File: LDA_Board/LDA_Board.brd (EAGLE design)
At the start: 47.5 x 68.4 mm, 65 parts, among them IC1 STM32F407ZET, IC3 IS62WV5121655T, K1 B3U-1000P, K2 B3U-1000P, U1 CJT1117-3.3-SOT223, Y1 27.12MHZ

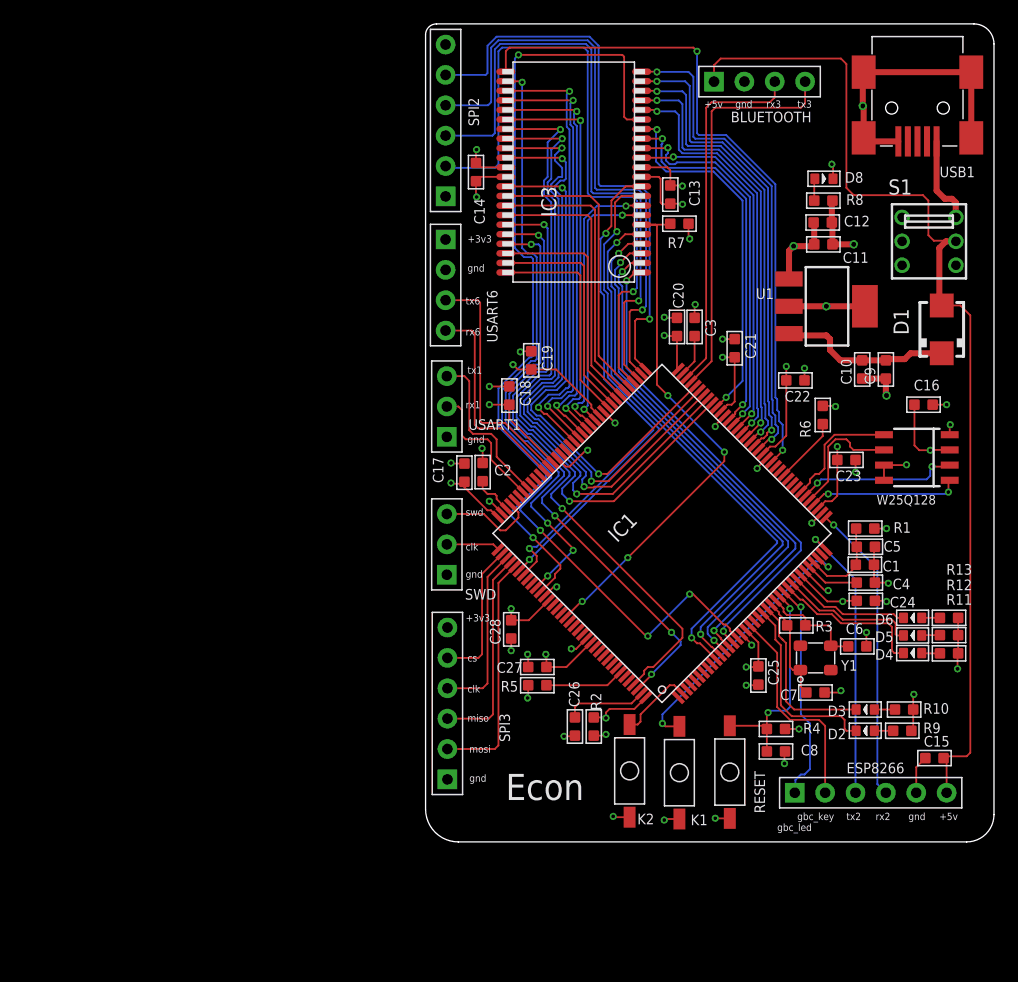
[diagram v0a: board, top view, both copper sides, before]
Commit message: 3D打印了盒子
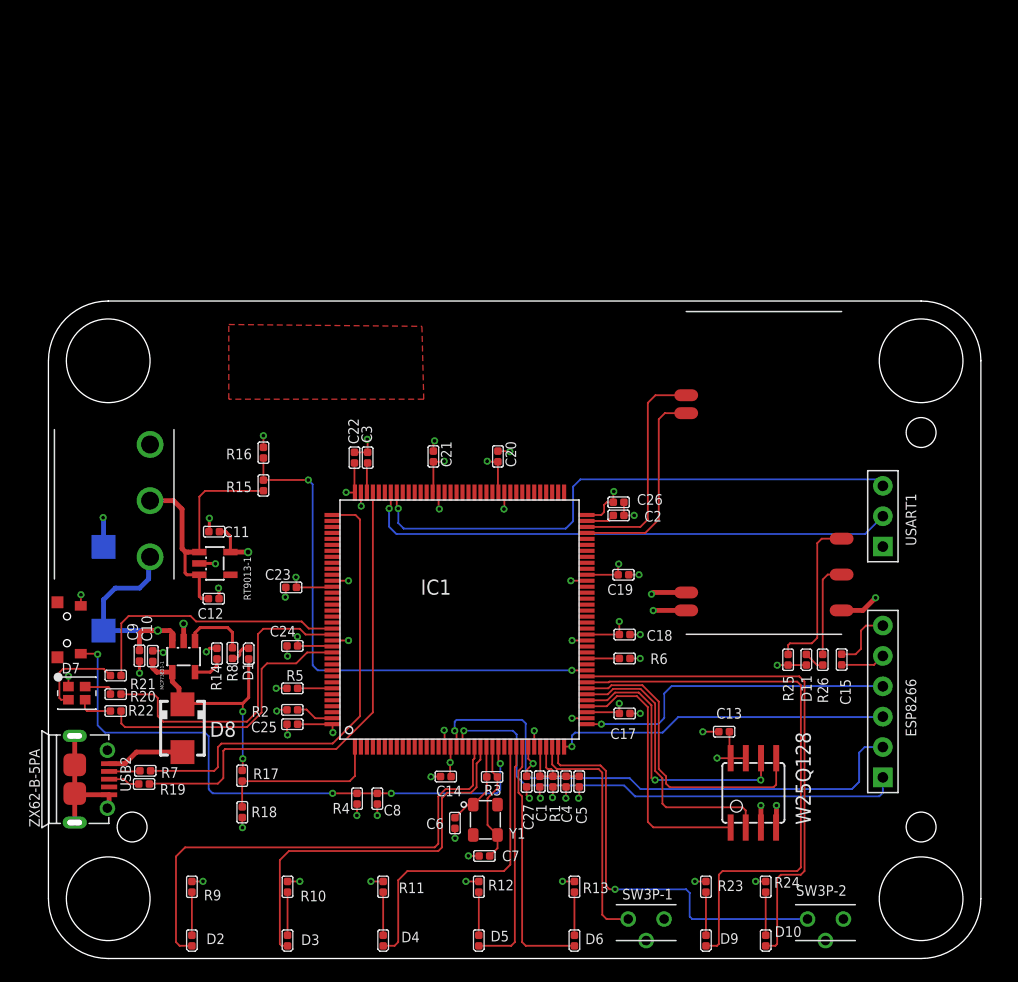
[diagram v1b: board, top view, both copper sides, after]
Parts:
- removed BLUETOOTH, USART6: 4p-2.54, Seeed-OPL-Connector:H4-2.54
- removed C16, C28: 0.5PF 50V, 1-LDA_Board:C0603
- removed IC3: IS62WV5121655T, 1-LDA_Board:TSOP-II-44
- removed K1, K2, RESET: B3U-1000P, 1-LDA_Board:SW2-SMD-3.0X6.0*2.5
- removed S1: 5.8X5.8SWITCH, 1-LDA_Board:2P2T
- removed SPI2, SPI3: 6p-2.54, Seeed-OPL-Connector:H6-2.54
- removed SWD: 3p-2.54, 1-LDA_Board:H3-2.54
- removed U1: CJT1117-3.3-SOT223, 1-LDA_Board:SOT-223
- removed USB1: ST-USB-002A, 1-LDA_Board:MINIUSB5+4P-SMD-0.8-90D
- added B-1: SIDE-BUTTON, 1-LDA_Board:SIDE-BUTTON
- added BATTERY-1: BATTERY, 1-LDA_Board:BATTERY
- added D10, D11, D9: BLUE-0402, 1-LDA_Board:LED-0402
- added D7: HSMF-C118, 1-LDA_Board:LED4-SMD-1210
- added HC05-1: BLUETOOTH, 1-LDA_Board:BLUETOOTH
- added MCP73831-1: MCP73831, 1-LDA_Board:SOT23-5
- added R14: 2k, 1-LDA_Board:R0402
- added R15, R16, R17, R25: 10k, 1-LDA_Board:R0402
- added R18: 20k, 1-LDA_Board:R0402
- added R19: 0R, 1-LDA_Board:R0402
- added R20, R21, R22, R23, R24: 510R, 1-LDA_Board:R0402
- added R26: 1.5k, 1-LDA_Board:R0402
- added RT9013-1: RT9013, 1-LDA_Board:SOT23-5
- added SW-1: SWITCH-3P, 1-LDA_Board:SWITCH-3P
- added SW3P-1, SW3P-2: LD-CCB-001, 1-LDA_Board:SW3-2.54-9.0X3.5X3.5+2.0MM
- added USB2: ZX62-B-5PA, 1-LDA_Board:MICRO-USB5+6P-SMD-0.65-AB
- C1, C13, C14, C2, C3: device 1-LDA_Board:C0603 -> 1-LDA_Board:C0402
- C10, C9: value 0.5PF 50V -> 4.7uf; device 1-LDA_Board:C0603 -> 1-LDA_Board:C0402
- C11: value 0.5PF 50V -> 1uf; device 1-LDA_Board:C0603 -> 1-LDA_Board:C0402
- C12: value 0.5PF 50V -> 10uf; device 1-LDA_Board:C0603 -> 1-LDA_Board:C0402
- C15, C17, C18, C19, C20, C21, C22, C23, C24, C25, C26, C27, C8: value 0.5PF 50V -> 104; device 1-LDA_Board:C0603 -> 1-LDA_Board:C0402
- C4: value 104 -> 10uf; device 1-LDA_Board:C0603 -> 1-LDA_Board:C0402
- C5: value 10uf -> 104; device 1-LDA_Board:C0603 -> 1-LDA_Board:C0402
- C6, C7: value 0.5PF 50V -> 22pf; device 1-LDA_Board:C0603 -> 1-LDA_Board:C0402
- D1: value SS14 -> BLUE-0402; device 1-LDA_Board:SMA -> 1-LDA_Board:LED-0402
- D2, D3, D4, D5, D6: value BLUE-0603 -> BLUE-0402; device Seeed-OPL-Diode:LED-0603 -> 1-LDA_Board:LED-0402
- D8: value BLUE-0603 -> SS14; device Seeed-OPL-Diode:LED-0603 -> 1-LDA_Board:SMA
- R1, R2: device 1-LDA_Board:R0603 -> 1-LDA_Board:R0402
- R10, R11, R12, R13, R9: value 1.1M 1/10W -> 510R; device 1-LDA_Board:R0603 -> 1-LDA_Board:R0402
- R3: value 1.1M 1/10W -> 1M; device 1-LDA_Board:R0603 -> 1-LDA_Board:R0402
- R4: value 1.1M 1/10W -> 10k; device 1-LDA_Board:R0603 -> 1-LDA_Board:R0402
- R5, R6, R7: value 10k -> 0R; device 1-LDA_Board:R0603 -> 1-LDA_Board:R0402
- R8: value 1.1M 1/10W -> 470R; device 1-LDA_Board:R0603 -> 1-LDA_Board:R0402
- W25Q128: device 1-LDA_Board:SOIC8 -> 1-LDA_Board:SOP08
- Y1: value 27.12MHZ -> 8MHZ
- moved D8 70.7 mm to (11.2, 19.3), turned to 270 degrees
- moved C9 66.9 mm to (7.61, 25.3)
- moved D1 64.0 mm to (16.8, 25.5)
- moved C10 64.0 mm to (8.73, 25.3), turned to 0 degrees
- moved R7 64.0 mm to (8.10, 15.7), turned to 90 degrees
- moved R8 62.3 mm to (15.4, 25.5), turned to 180 degrees
- moved R9 60.8 mm to (12.0, 6.00), turned to 0 degrees
- moved C12 59.9 mm to (13.8, 30.1), turned to 270 degrees
- moved D2 59.0 mm to (12.0, 1.50), turned to 270 degrees
- moved C11 56.3 mm to (13.9, 35.7), turned to 270 degrees
- moved R10 53.7 mm to (20.0, 6.00), turned to 0 degrees
- moved D3 52.0 mm to (20.0, 1.50), turned to 270 degrees
- moved R11 51.2 mm to (28.0, 6.00), turned to 0 degrees
- moved C14 50.6 mm to (33.2, 15.2), turned to 90 degrees
- moved D4 50.4 mm to (28.0, 1.50), turned to 270 degrees
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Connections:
- removed net FSMC_A0: IC1.10, IC3.5
- removed net FSMC_A1: IC1.11, IC3.4
- removed net FSMC_A10: IC1.56, IC3.19
- removed net FSMC_A11: IC1.57, IC3.18
- removed net FSMC_A12: IC1.87, IC3.28
- removed net FSMC_A13: IC1.88, IC3.27
- removed net FSMC_A14: IC1.89, IC3.26
- removed net FSMC_A15: IC1.90, IC3.25
- removed net FSMC_A16: IC1.80, IC3.42
- removed net FSMC_A17: IC1.81, IC3.43
- removed net FSMC_A18: IC1.82, IC3.44
- removed net FSMC_A2: IC1.12, IC3.3
- removed net FSMC_A3: IC1.13, IC3.2
- removed net FSMC_A4: IC1.14, IC3.1
- removed net FSMC_A5: IC1.15, IC3.24
- removed net FSMC_A6: IC1.50, IC3.23
- removed net FSMC_A7: IC1.53, IC3.22
- removed net FSMC_A8: IC1.54, IC3.21
- removed net FSMC_A9: IC1.55, IC3.20
- removed net FSMC_D0: IC1.85, IC3.7
- removed net FSMC_D1: IC1.86, IC3.8
- removed net FSMC_D10: IC1.66, IC3.31
- removed net FSMC_D11: IC1.67, IC3.32
- removed net FSMC_D12: IC1.68, IC3.35
- removed net FSMC_D13: IC1.77, IC3.36
- removed net FSMC_D14: IC1.78, IC3.37
- removed net FSMC_D15: IC1.79, IC3.38
- removed net FSMC_D2: IC1.114, IC3.9
- removed net FSMC_D3: IC1.115, IC3.10
- removed net FSMC_D4: IC1.58, IC3.13
- removed net FSMC_D5: IC1.59, IC3.14
- removed net FSMC_D6: IC1.60, IC3.15
- removed net FSMC_D7: IC1.63, IC3.16
- removed net FSMC_D8: IC1.64, IC3.29
- removed net FSMC_D9: IC1.65, IC3.30
- removed net FSMC_NBL0: IC1.141, IC3.39
- removed net FSMC_NBL1: IC1.142, IC3.40
- removed net FSMC_NE3: IC1.125, IC3.6, R7.2
- removed net FSMC_NOE: IC1.118, IC3.41
- removed net FSMC_NWE: IC1.119, IC3.17
- removed net RX6: IC1.97, USART6.4
- removed net SPI2_CLK: IC1.74, SPI2.4
- removed net SPI2_CS: IC1.73, SPI2.5
- removed net SPI2_MISO: IC1.75, SPI2.3
- removed net SPI2_MOSI: IC1.76, SPI2.2
- removed net SPI3_CLK: IC1.111, SPI3.4
- removed net SPI3_CS: IC1.110, SPI3.5
- removed net SPI3_MISO: IC1.112, SPI3.3
- removed net SPI3_MOSI: IC1.113, SPI3.2
- removed net TX6: IC1.96, USART6.3
- new net +3.7V: C12.2, R15.1, RT9013-1.1, RT9013-1.3, SW-1.P$2
- new net BATTERY: BATTERY-1.P$1, C9.2, MCP73831-1.3, SW-1.P$3
- new net LED6: D9.-, IC1.44
- new net LED7: D10.-, IC1.45
- new net LED_B: IC1.129, R20.1
- new net LED_G: IC1.132, R22.1
- new net LED_R: IC1.128, R21.1
- new net LI_CHARGE: IC1.1, R17.2, R18.1
- new net LI_QUANTITY: IC1.46, R15.2, R16.1
- new net N$12: D7.2, R21.2
- new net N$16: D1.-, R8.1
- new net N$17: HC05-1.P$26, R25.1
- new net N$18: D7.3, R22.2
- new net N$19: HC05-1.P$24, R26.1
- new net N$20: D11.+, R26.2
- new net N$24: D9.+, R23.2
- new net N$25: D10.+, R24.2
- new net USB_D+: R19.1, USB2.3
- new net USB_D-: R7.1, USB2.2
- new net VBUS: D8.A, USB2.1
- net +3V3: now also C11.1, C13.2, C14.2, C15.1, ESP8266.6, HC05-1.P$12, R23.1, R24.1, RT9013-1.5, SW3P-1.1; no longer C11.2, C12.2, C13.1, C14.1, C16.1, C28.2, IC3.11, IC3.33, K1.1, R7.1, R8.1, SPI2.6, SPI3.6, U1.2, U1.TER, USART6.1
- net +5V: now also C10.2, D1.+, D8.C, MCP73831-1.4, R17.1; no longer BLUETOOTH.1, C15.1, D1.A, ESP8266.6, S1.2.1
- net CLK: now also R7.2; no longer SWD.2
- net GBC_LED: now also IC1.19; no longer IC1.26
- net GND: now also B-1.P$1, BATTERY-1.P$2, C1.2, C11.2, C13.1, C14.1, C2.2, C3.2, C6.1, C7.1, C8.1, D11.-, D7.1, HC05-1.P$13, HC05-1.P$22, MCP73831-1.2, R14.2, R16.2, R18.2, R25.2, RT9013-1.2, SW3P-2.1, USB2.5, USB2.P1, USB2.P2, USB2.P3, USB2.P4, USB2.P5, USB2.P6; no longer BLUETOOTH.2, C1.1, C11.1, C13.2, C14.2, C16.2, C2.1, C28.1, C3.1, C6.2, C7.2, C8.2, D8.-, IC3.12, IC3.34, K2.1, RESET.2, SPI2.1, SPI3.1, SWD.1, U1.1, USART6.2, USB1.5, USB1.P$1, USB1.P$2, USB1.P$3, USB1.P$4
- net KEY1: now also IC1.35, SW3P-2.2; no longer IC1.2, K2.2
- net N$10: now also D7.4, R20.2; no longer S1.1.1, USB1.1
- net N$11: now also MCP73831-1.5, R14.1; no longer D8.+, R8.2
- net N$2: now also C2.1; no longer C3.2
- net N$3: now also C3.1; no longer C2.2
- net N$4: now also IC1.48; no longer IC1.47
- net N$5: now also C1.1; no longer C1.2
- net N$6: now also MCP73831-1.1, R8.2; no longer C10.2, C9.2, D1.C, U1.3
- net OSC_IN: now also C6.2; no longer C7.1
- net OSC_OUT: now also C7.2; no longer C6.1
- net RESET: now also B-1.P$2, C8.2; no longer C8.1, RESET.1
- net RX3: now also HC05-1.P$1; no longer BLUETOOTH.3
- net SWD: now also R19.2; no longer SWD.3
- net TX3: now also HC05-1.P$2; no longer BLUETOOTH.4
- net WK_UP: now also SW3P-1.2; no longer K1.2
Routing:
- net FSMC_NWE: track 68.0 -> 0.00 mm, vias 2 -> 0
- net FSMC_A5: track 67.7 -> 0.00 mm, vias 4 -> 0
- net +5V: track 87.2 -> 20.0 mm, vias 0 -> 2
- net FSMC_A6: track 57.1 -> 0.00 mm, vias 2 -> 0
- net FSMC_D8: track 56.4 -> 0.00 mm, vias 2 -> 0
- net SPI2_MOSI: track 54.9 -> 0.00 mm, vias 1 -> 0
- net FSMC_D9: track 53.8 -> 0.00 mm, vias 2 -> 0
- net FSMC_NBL0: track 52.7 -> 0.00 mm, vias 2 -> 0
- net SPI2_MISO: track 52.6 -> 0.00 mm, vias 1 -> 0
- net FSMC_D10: track 51.8 -> 0.00 mm, vias 2 -> 0
- net FSMC_NBL1: track 51.6 -> 0.00 mm, vias 4 -> 0
- net SPI2_CLK: track 50.3 -> 0.00 mm, vias 1 -> 0
- net FSMC_D11: track 48.9 -> 0.00 mm, vias 2 -> 0
- net SPI2_CS: track 48.1 -> 0.00 mm, vias 1 -> 0
- net LED6: track 0.00 -> 47.4 mm
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- added copper zone on layer 1, net N$21
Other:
- board size 47.5 x 68.4 mm -> 78 x 55 mm
- board text added: "5个手势显示灯"
- board text added: "ECON-TECH"
- board text added: "usb充电口"
- board text added: "侧边 复位键"
- board text added: "拓展串口、wifi"
- board text added: "电源拨码 开关"
- board text added: "电源状态 指示灯"
- board text added: "蓝牙"
- board text added: "训练和工作按键 训练和工作指示灯"
- board text removed: "+3v3"
- board text removed: "+5v"
- board text removed: "Econ"
- board text removed: "clk"
- board text removed: "cs"
- board text removed: "gbc_key"
- board text removed: "gbc_led"
- board text removed: "gnd"
- board text removed: "miso"
- board text removed: "mosi"
- board text removed: "rx1"
- board text removed: "rx2"
- board text removed: "rx3"
- board text removed: "rx6"
- board text removed: "swd"
- board text removed: "tx1"
- board text removed: "tx2"
- board text removed: "tx3"
- board text removed: "tx6"
